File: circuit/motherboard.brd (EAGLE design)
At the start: 155.2 x 104.8 mm, 16 parts, among them J1 XF2L-2235-1, J2 XF2L-2235-1, T1 BC337

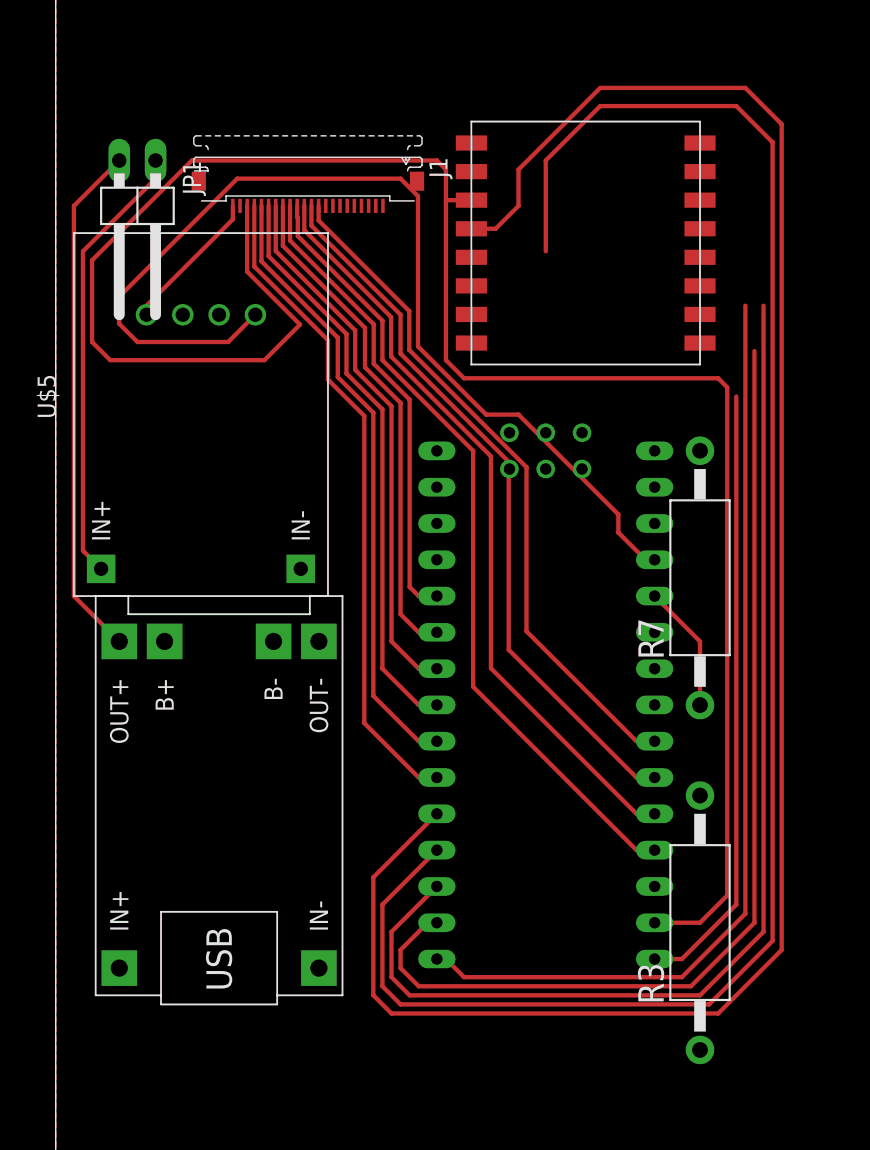
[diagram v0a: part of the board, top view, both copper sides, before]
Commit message: Motherboard complete!
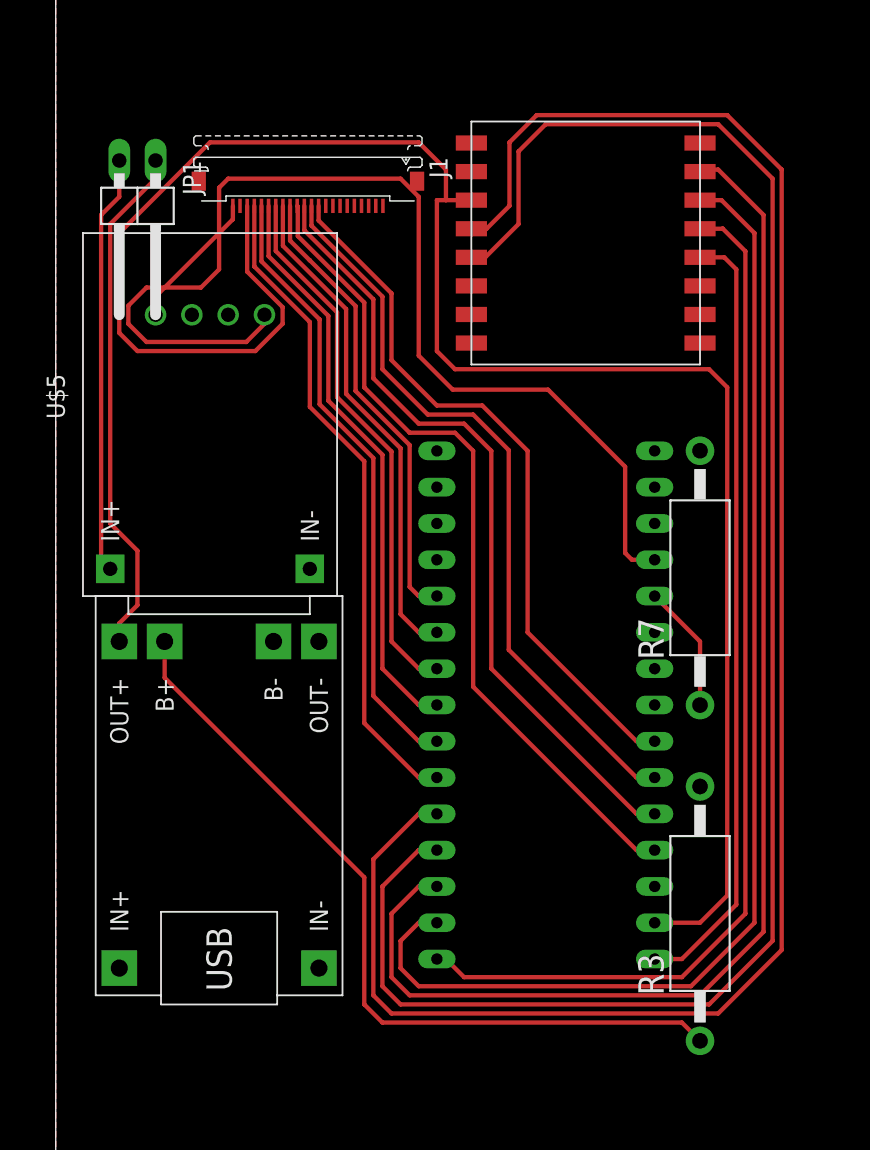
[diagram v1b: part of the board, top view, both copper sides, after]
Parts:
- U$1: device Arduino-clone:NANO -> Arduino-clone-nano-minimal:NANO
- moved R3 0.63 mm to (52.7, 10.8)
- moved U$5 0.63 mm to (18.4, 45.7)
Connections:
- net GND: now also U$4.P$2
- net N$1: now also U$3.OUT+; no longer U$5.IN+
- net N$15: now also U$5.IN+; no longer U$3.OUT+
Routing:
- net N$16: track 0.00 -> 55.7 mm
- net N$5: track 71.7 -> 85.1 mm
- net N$6: track 79.9 -> 92.8 mm
- net N$2: track 42.9 -> 54.6 mm
- net N$4: track 66.5 -> 74.1 mm
- net N$15: track 36.3 -> 29.4 mm
- net +5V: track 71.6 -> 77.4 mm
- net N$1: track 31.2 -> 36.3 mm
- net +3V3: track 136.6 -> 133.2 mm
- net N$7: track 121.5 -> 124.4 mm
- net N$35: track 47.9 -> 49.8 mm
- net N$34: track 50.7 -> 52.6 mm
- net N$33: track 53.4 -> 55.3 mm
- net N$32: track 56.2 -> 58.1 mm
- net N$8: track 131.6 -> 130.0 mm
